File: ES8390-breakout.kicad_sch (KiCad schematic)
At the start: 65 parts, among them CN1 Conn_01x14_Pin, CN2 PJ-327A, CN3 PJ-327A, J1 PJ-603A, J2 Conn_01x02_Pin, J3 Conn_01x02_Pin, U1 TLV9062, U2 LP5907MFX-3.0, U3 ES8390, U4 IM68A130AXTMA1, U5 MAX98306xDT

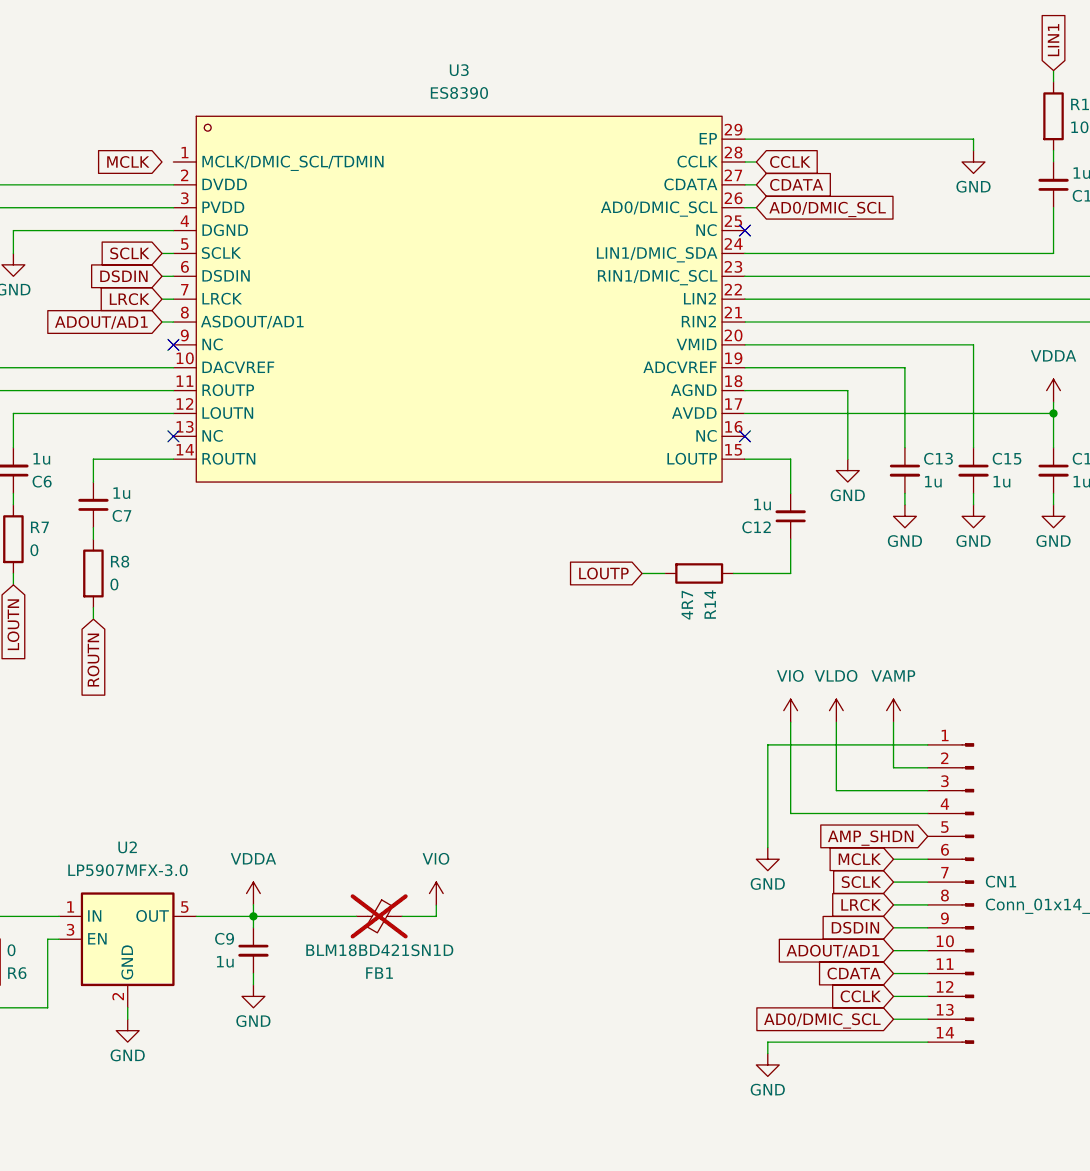
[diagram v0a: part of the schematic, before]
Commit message: first layout done
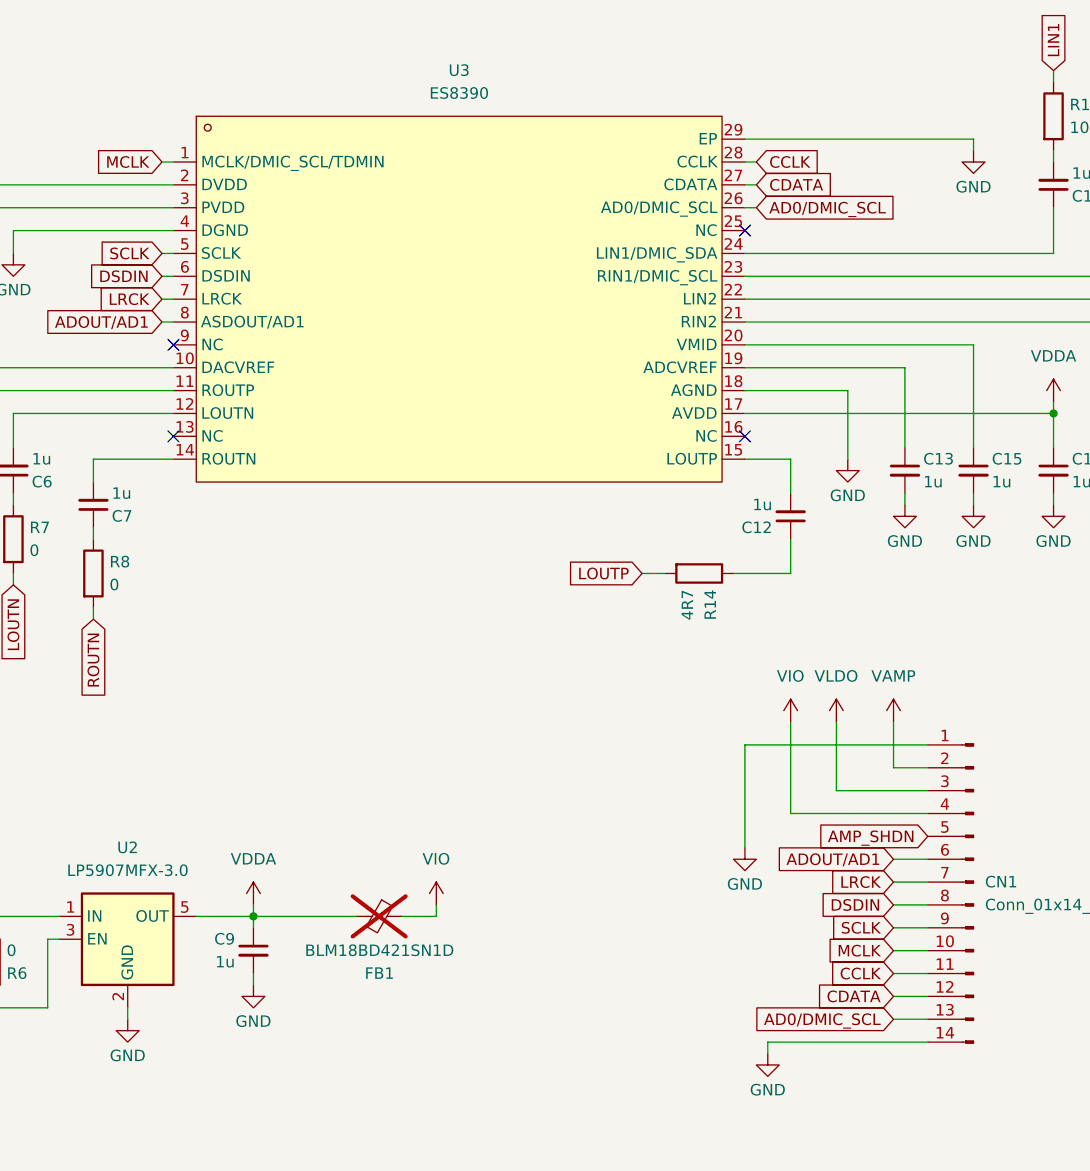
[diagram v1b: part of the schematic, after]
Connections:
- net ADOUT/AD1: now also CN1.6 (Pin_6); no longer CN1.10 (Pin_10)
- net CCLK: now also CN1.11 (Pin_11); no longer CN1.12 (Pin_12)
- net CDATA: now also CN1.12 (Pin_12); no longer CN1.11 (Pin_11)
- net DSDIN: now also CN1.8 (Pin_8); no longer CN1.9 (Pin_9)
- net LRCK: now also CN1.7 (Pin_7); no longer CN1.8 (Pin_8)
- net MCLK: now also CN1.10 (Pin_10), U3.1 (MCLK/DMIC_SCL/TDMIN); no longer CN1.6 (Pin_6)
- net SCLK: now also CN1.9 (Pin_9); no longer CN1.7 (Pin_7)
